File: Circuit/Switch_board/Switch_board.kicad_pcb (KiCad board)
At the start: 2 copper layers, 27 parts, among them J1 switch_mode, J2 switch, P1 XT30, Q1 2N7002, Q2 2N7002, Q3 2N7002, Q4 2N7002, U1 DRV5023

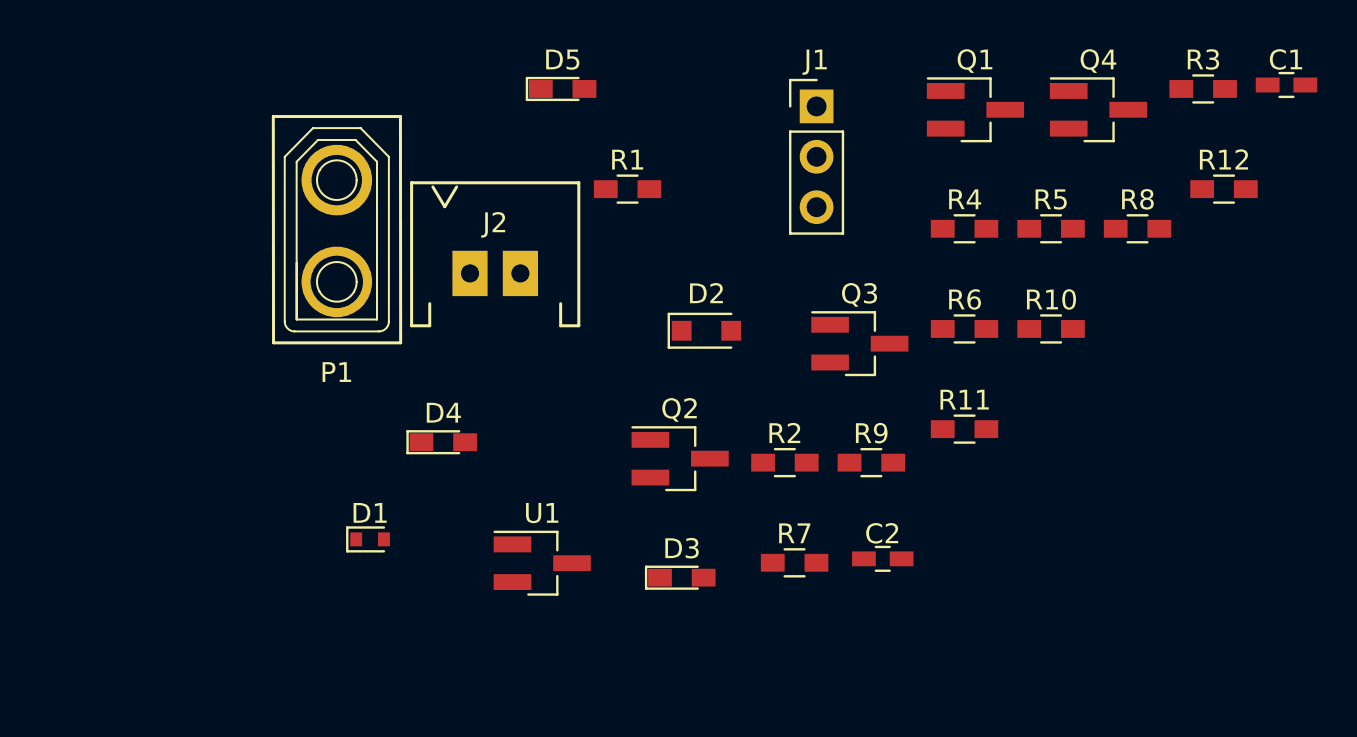
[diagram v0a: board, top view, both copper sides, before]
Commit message: pcb layout of Switch_board was drafted
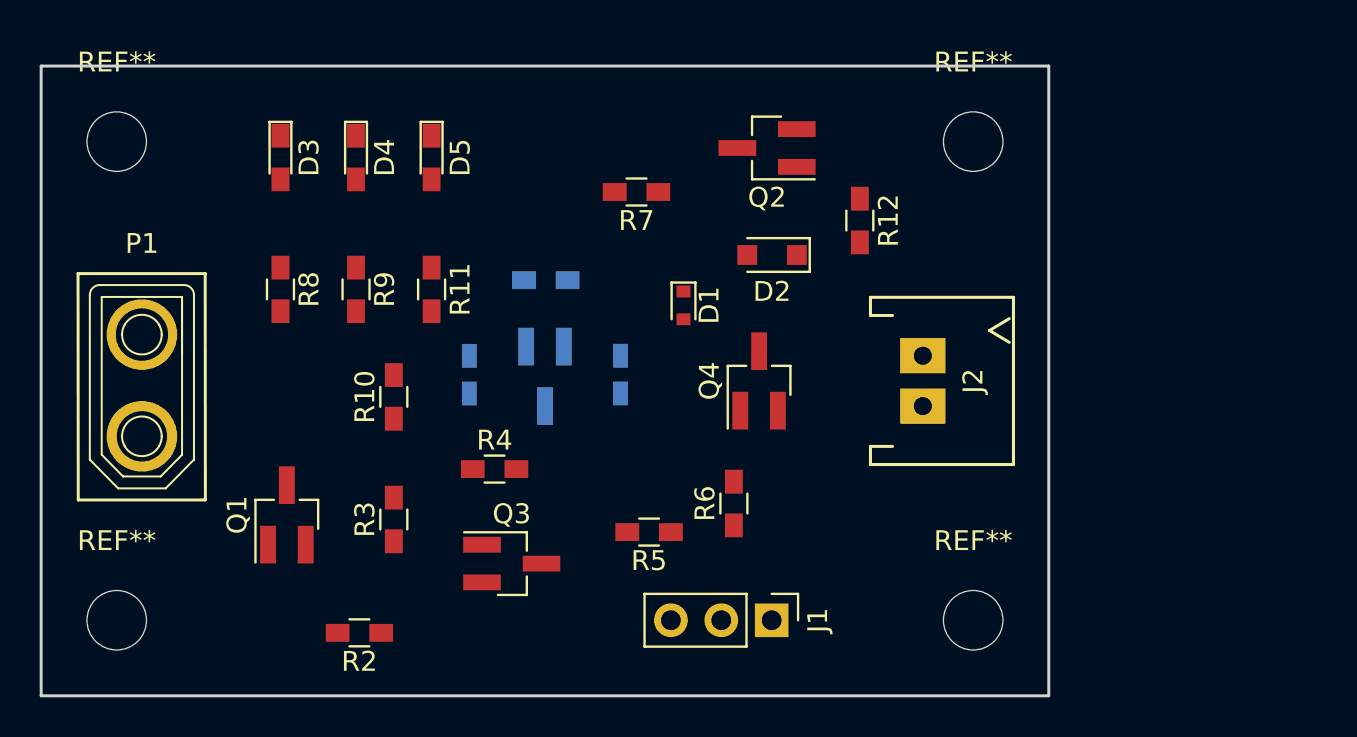
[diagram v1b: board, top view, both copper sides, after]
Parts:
- added REF**: MountingHole_3mm, Mounting_Holes:MountingHole_3mm, F.Cu at (143.5, 135.9)
- added REF**: MountingHole_3mm, Mounting_Holes:MountingHole_3mm, F.Cu at (143.5, 111.8)
- added REF**: MountingHole_3mm, Mounting_Holes:MountingHole_3mm, F.Cu at (186.7, 111.8)
- added REF**: MountingHole_3mm, Mounting_Holes:MountingHole_3mm, F.Cu at (186.7, 135.9)
- C1, C2, R1, U1: moved to B.Cu
- moved R3 46.2 mm to (157.5, 130.8), turned to 90 degrees
- moved C1 43.7 mm to (161.3, 123.5), turned to 270 degrees
- moved R8 43.3 mm to (151.8, 119.2), turned to 270 degrees
- moved Q1 40.3 mm to (152.1, 130.6), turned to 90 degrees
- moved R10 33.3 mm to (157.5, 124.6), turned to 90 degrees
- moved D3 29.3 mm to (151.8, 112.6), turned to 270 degrees
- moved R11 27.8 mm to (159.4, 119.2), turned to 270 degrees
- moved R9 27.4 mm to (155.6, 119.2), turned to 270 degrees
- moved R4 26.6 mm to (162.6, 128.3)
- moved J1 26.0 mm to (176.5, 135.9), turned to 270 degrees
- moved R5 25.4 mm to (170.3, 131.4), turned to 180 degrees
- moved R2 23.1 mm to (155.7, 136.5), turned to 180 degrees
- moved J2 22.2 mm to (184.2, 123.8), turned to 270 degrees
- moved Q4 21.9 mm to (175.9, 123.8), turned to 90 degrees
- moved Q3 20.8 mm to (163.4, 133.0)
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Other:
- board outline added: 50.8 x 31.7 mm
